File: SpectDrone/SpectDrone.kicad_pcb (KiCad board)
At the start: 2 copper layers, 215 x 71.1 mm, 75 parts, among them J1 Camera, J2 GPS, J4 BME280, J5-1 BNO055-1, J5-2 BNO055-2, Q1 FDN340P, Q2 FDN340P, SW0 SW_Push, SW1 SW_Push, SW10 SW_Push, SW2 SW_Push, SW3 SW_Push, SW4 SW_Push, SW5 SW_Push, SW6 SW_Push, SW7 SW_Push, SW8 SW_Push, SW9 SW_Push, U1 C12666MA, U2 C12666MA, U3 LM7805_TO220, U4 MCP112-300E/TO, U5 MCP112-300E/TO, U6 LM7805_TO220, U7 Teensy3.2

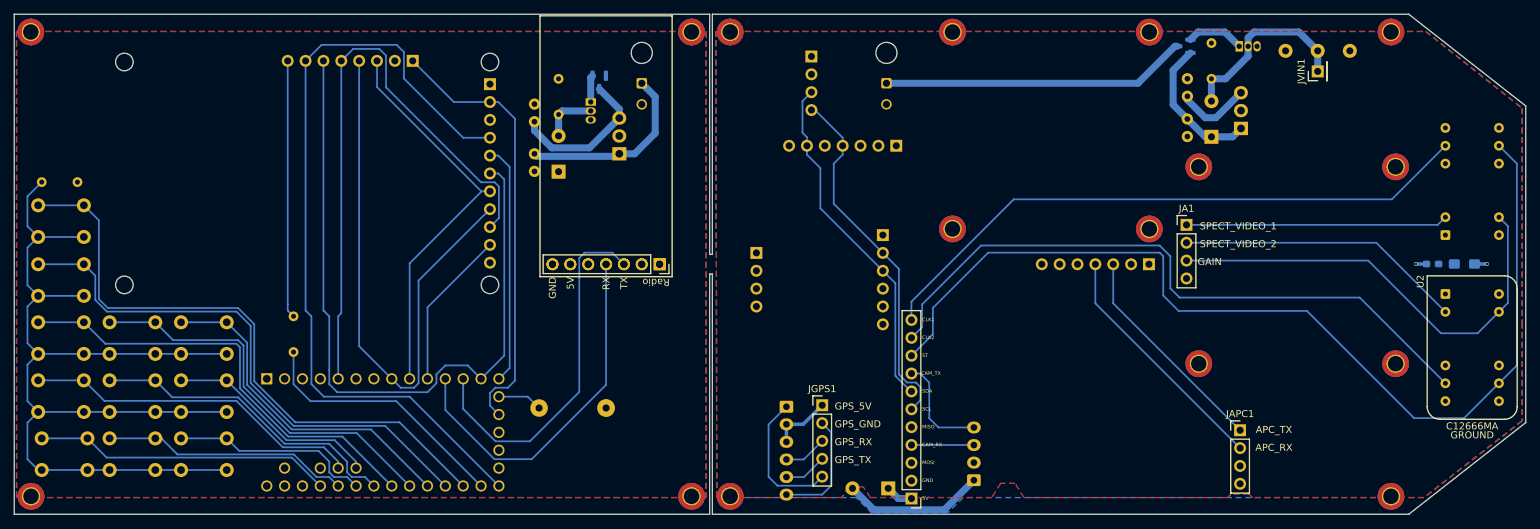
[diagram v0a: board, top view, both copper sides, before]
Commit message: SpectDrone Development
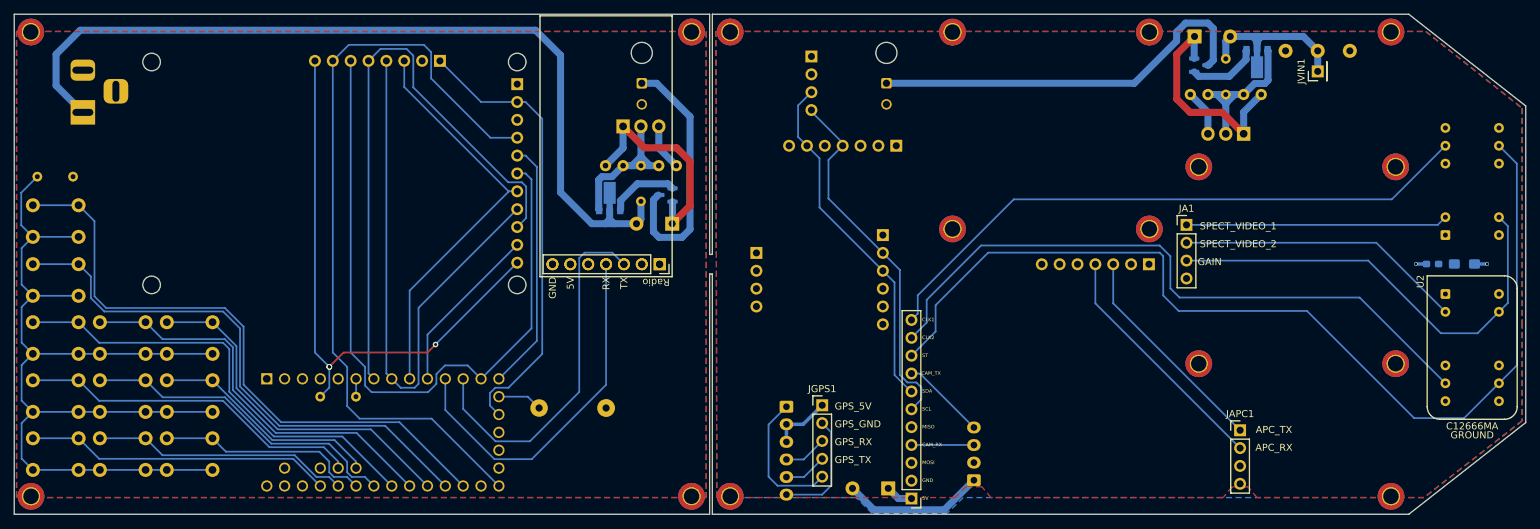
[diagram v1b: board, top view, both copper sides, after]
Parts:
- added J3: Barrel_Jack, Connector_BarrelJack:BarrelJack_Horizontal, B.Cu at (52.1, 88.3)
- U4, U5: footprint Package_TO_SOT_THT:TO-92_Inline -> Package_TO_SOT_SMD:SOT-89-3
- moved C6 21.1 mm to (136.5, 95.8), turned to 180 degrees
- moved Q2 18.6 mm to (135.0, 100.0), turned to 180 degrees
- moved D2 17.8 mm to (135.9, 104.1), turned to 180 degrees
- moved R2 17.0 mm to (131.5, 100.9)
- moved D1 14.5 mm to (210.2, 77.5), turned to 0 degrees
- moved U5 13.9 mm to (127.0, 100.4), turned to 90 degrees
- moved C5 12.6 mm to (128.9, 95.8), turned to 180 degrees
- moved R3 10.9 mm to (90.9, 128.7), turned to 180 degrees
- moved C3 9.99 mm to (217.2, 85.7), turned to 0 degrees
- moved U6 3.94 mm to (128.9, 90.2), turned to 0 degrees
- moved JD1 3.87 mm to (102.9, 80.9)
- moved H19 3.87 mm to (61.9, 112.8)
- moved H20 3.87 mm to (61.9, 81.1)
- moved H17 3.87 mm to (113.9, 81.1)
- moved H18 3.87 mm to (113.9, 112.8)
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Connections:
- net /7-12V renamed /7-12V1
- C5 pad 2: /VBAT2 -> /7-12V2
- C6 pad 1: /VOUT2 -> /5V4
- D2 pad 1: /5V4 -> /7-12V2
- JD1 pad 8: Net-(JD1-Pad8) -> /BKL
- Q2 pad 2: /5V4 -> /7-12V2
- Q2 pad 3: /VOUT2 -> /VBAT2
- R3 pad 2: Net-(JD1-Pad8) -> /BKL
- U6 pad 1: /VBAT2 -> /7-12V2
- U6 pad 3: /VOUT2 -> /5V4
- U7 pad 21: /LED -> unconnected-(U7-Pad21)
- U7 pad 5: /D/C -> unconnected-(U7-Pad5)
- U7 pad 6: unconnected-(U7-Pad6) -> /LED
- U7 pad 7: unconnected-(U7-Pad7) -> /D/C
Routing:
- net /VIN2: track 7.83 -> 123.0 mm
- net /BKL: track 0.00 -> 82.0 mm, vias 0 -> 4
- net Net-(JD1-Pad8): track 36.7 -> 0.00 mm
- net /LED: track 37.2 -> 2.55 mm
- net /7-12V2: track 0.00 -> 31.3 mm
- net /GND2: track 0.00 -> 22.8 mm
- net /GND1: track 3.37 -> 26.2 mm
- net /VOUT2: track 21.4 -> 0.00 mm
- net /VBAT: track 43.5 -> 56.8 mm
- net /7-12V1: track 20.4 -> 31.2 mm
- net /VBAT2: track 26.1 -> 36.4 mm
- net /5V4: track 0.00 -> 6.63 mm
- net Net-(Q2-Pad1): track 3.84 -> 9.96 mm
- net /5V3: track 30.9 -> 26.9 mm
- net /VIN1: track 26.6 -> 22.9 mm
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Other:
- board text removed: "BKL"
